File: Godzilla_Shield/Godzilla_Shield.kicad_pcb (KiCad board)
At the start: 2 copper layers, 9 parts, among them J1 6V, J2 12V, J3 Linha_Esq, J4 Linha_Dir, J5 Obstaculo, J6 Motor_Esq, J7 Motor_Dir, J8 Ultrassom

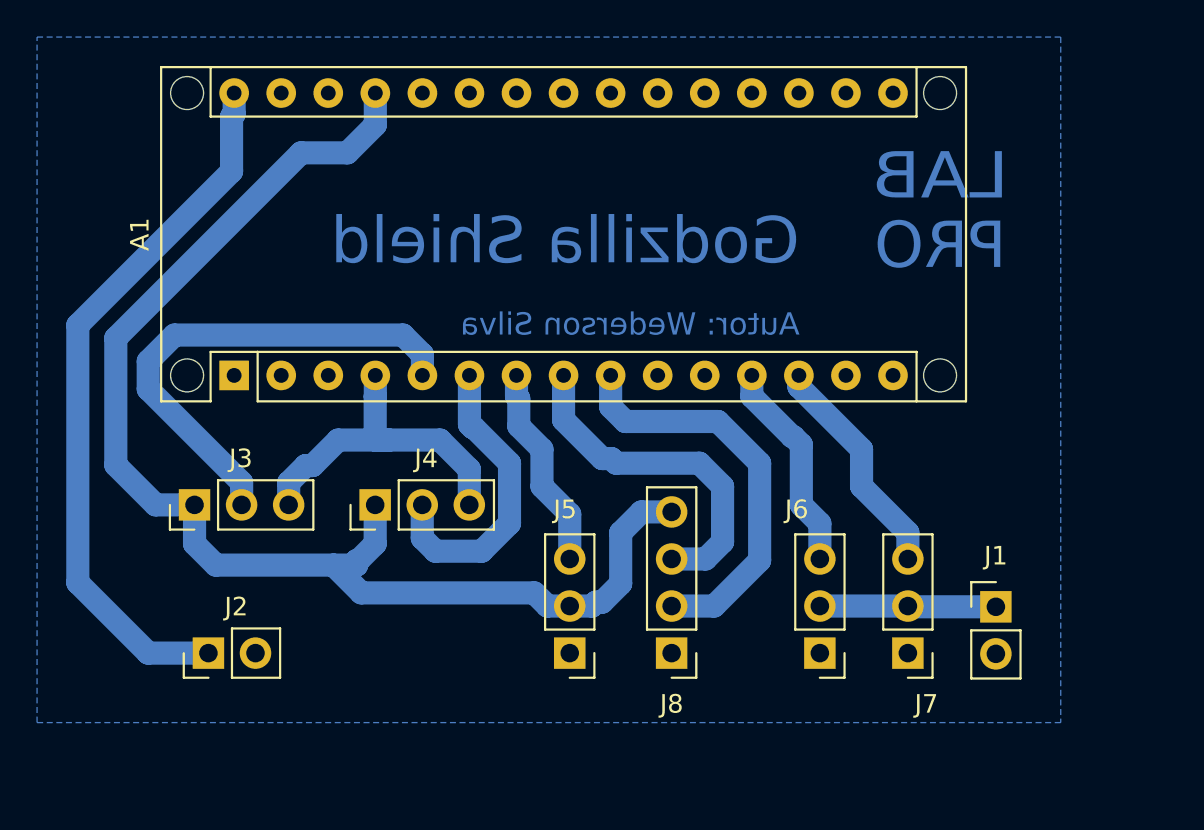
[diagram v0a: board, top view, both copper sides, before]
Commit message: Adiciona a versão 2 da placa
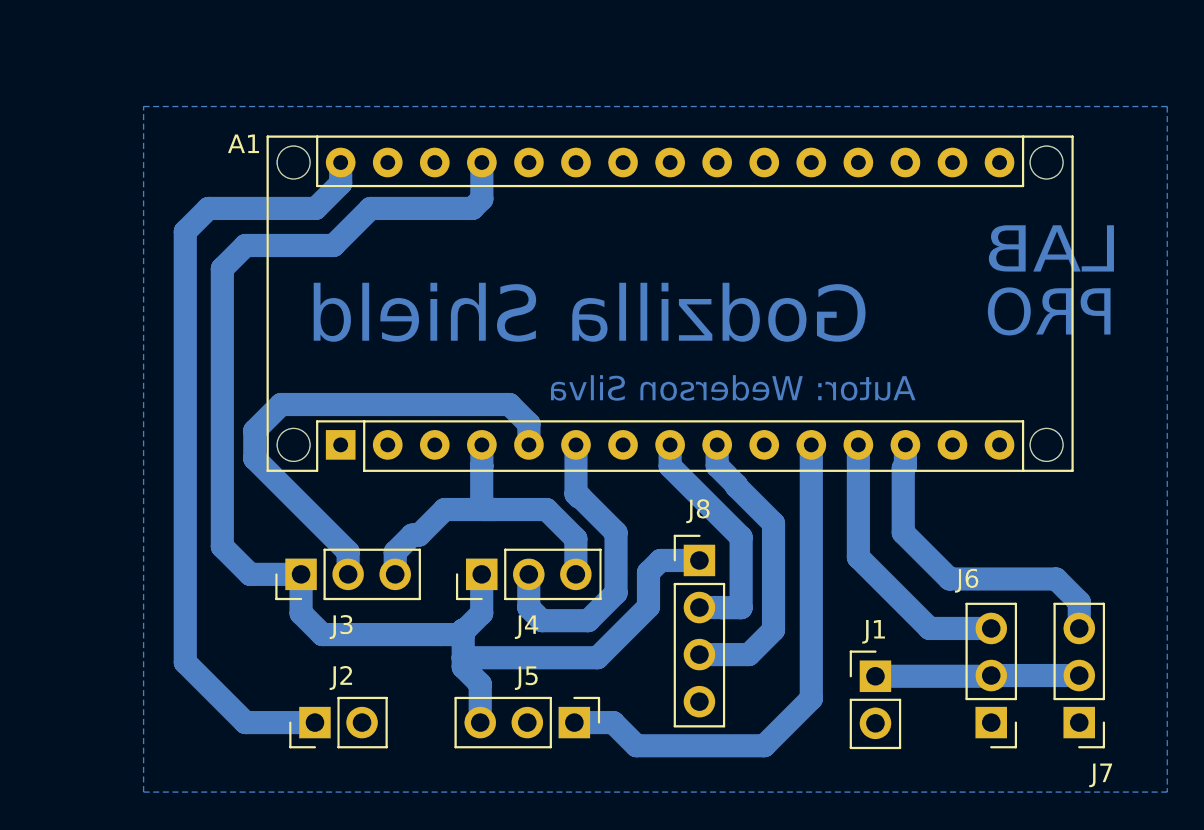
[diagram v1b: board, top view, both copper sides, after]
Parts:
- moved J6 9.98 mm to (228.5, 164.0)
- moved J7 9.98 mm to (233.2, 164.0)
- moved J1 7.50 mm to (222.2, 161.5)
- moved A1 6.86 mm to (193.4, 149.0)
- moved J2 6.86 mm to (192.0, 164.0)
- moved J3 6.86 mm to (191.2, 156.0)
- moved J4 6.86 mm to (201.0, 156.0)
- moved J8 5.22 mm to (212.8, 155.2), turned to 0 degrees
- moved J5 3.76 mm to (206.0, 164.0), turned to 270 degrees
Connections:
- J5 pad 1: /GND -> Net-(A1-Pad11)
- J5 pad 2: /5V -> /GND
- J5 pad 3: Net-(A1-Pad7) -> /5V
- J8 pad 1: /GND -> /5V
- J8 pad 2: /ECHO -> /TRIG
- J8 pad 3: /TRIG -> /ECHO
- J8 pad 4: /5V -> /GND
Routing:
- net Net-(A1-Pad11): track 0.00 -> 28.1 mm
- net Net-(A1-Pad7): track 11.1 -> 0.00 mm
- net /ECHO: track 22.0 -> 15.8 mm
- net /TRIG: track 18.6 -> 12.6 mm
- net Net-(A1-Pad13): track 12.3 -> 17.3 mm
- net Net-(A1-Pad30): track 38.5 -> 42.2 mm
- net Net-(A1-Pad12): track 11.5 -> 14.8 mm
- net /5V: track 70.4 -> 73.6 mm
- net /6V: track 9.52 -> 11.0 mm
